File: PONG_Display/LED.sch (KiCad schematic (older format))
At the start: 4 parts, among them J1 LED_Display_Conn, U1 PC817

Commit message: layout v1
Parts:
- C1: footprint Capacitor_SMD:C_1206_3216Metric_Pad1.42x1.75mm_HandSolder -> Capacitor_SMD:C_0603_1608Metric_Pad1.05x0.95mm_HandSolder
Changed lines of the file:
@@
 EESchema Schematic File Version 4
-LIBS:PONG_Display-cache
 EELAYER 30 0
 EELAYER END
@@
 F 0 "C1" H 3515 2996 50  0000 L CNN
 F 1 "100n" H 3515 2905 50  0000 L CNN
-F 2 "Capacitor_SMD:C_1206_3216Metric_Pad1.42x1.75mm_HandSolder" H 3438 2800 50  0001 C CNN
+F 2 "Capacitor_SMD:C_0603_1608Metric_Pad1.05x0.95mm_HandSolder" H 3438 2800 50  0001 C CNN
 F 3 "~" H 3400 2950 50  0001 C CNN
 	1    3400 2950

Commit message: l
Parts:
- R1: footprint Resistor_SMD:R_1206_3216Metric_Pad1.42x1.75mm_HandSolder -> Resistor_SMD:R_0603_1608Metric_Pad1.05x0.95mm_HandSolder
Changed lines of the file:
@@
 F 0 "R1" V 1993 2550 50  0000 C CNN
 F 1 "180R" V 2084 2550 50  0000 C CNN
-F 2 "Resistor_SMD:R_1206_3216Metric_Pad1.42x1.75mm_HandSolder" V 2130 2550 50  0001 C CNN
+F 2 "Resistor_SMD:R_0603_1608Metric_Pad1.05x0.95mm_HandSolder" V 2130 2550 50  0001 C CNN
 F 3 "~" H 2200 2550 50  0001 C CNN
 	1    2200 2550

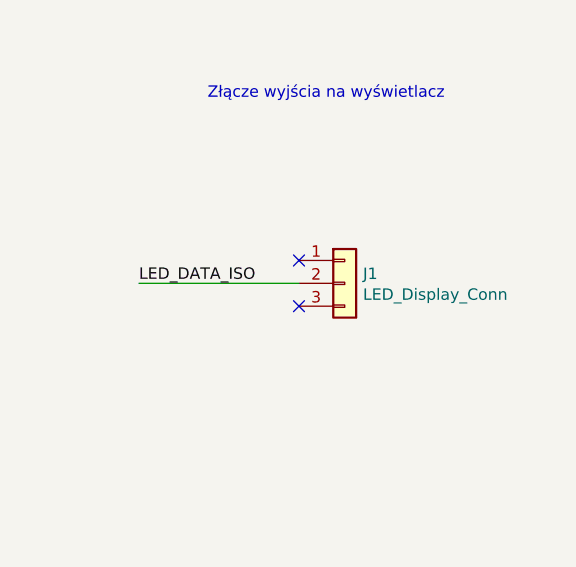
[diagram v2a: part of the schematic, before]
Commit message: layout4
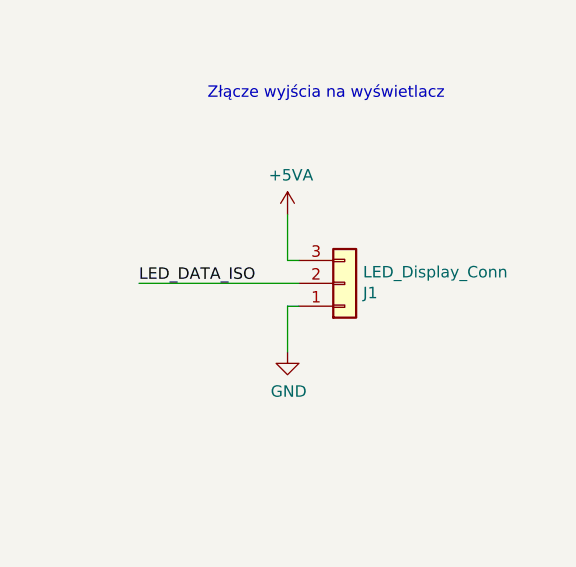
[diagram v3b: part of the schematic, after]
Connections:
- net GND: now also J1.1 (Pin_1)
- net +5VA: now reaches J1.3 (Pin_3)
- no-connect marks 2 -> 0
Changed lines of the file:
@@
 F 3 "~" H 8850 2800 50  0001 C CNN
 	1    8850 2800
-	1    0    0    -1
+	1    0    0    1
 $EndComp
 Text Notes 7750 7500 0    50   ~ 0
@@
 	1    0    0    -1
 $EndComp
-NoConn ~ 8650 2700
-NoConn ~ 8650 2900
+$Comp
+L power:GND #PWR0109
+U 1 1 5EB33F3E
+P 8600 3100
+F 0 "#PWR0109" H 8600 2850 50  0001 C CNN
+F 1 "GND" H 8605 2927 50  0000 C CNN
+F 2 "" H 8600 3100 50  0001 C CNN
+F 3 "" H 8600 3100 50  0001 C CNN
+	1    8600 3100
+	1    0    0    -1
+$EndComp
+Wire Wire Line
+	8600 2500 8600 2700
+Wire Wire Line
+	8600 2700 8650 2700
+Wire Wire Line
+	8600 3100 8600 2900
+Wire Wire Line
+	8600 2900 8650 2900
+$Comp
+L power:+5VA #PWR0110
+U 1 1 5EA4877F
+P 8600 2500
+F 0 "#PWR0110" H 8600 2350 50  0001 C CNN
+F 1 "+5VA" H 8615 2673 50  0000 C CNN
+F 2 "" H 8600 2500 50  0001 C CNN
+F 3 "" H 8600 2500 50  0001 C CNN
+	1    8600 2500
+	1    0    0    -1
+$EndComp
 $EndSCHEMATC

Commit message: laayout6
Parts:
- J1: footprint TerminalBlock:TerminalBlock_bornier-3_P5.08mm -> TerminalBlock_RND:TerminalBlock_RND_205-00002_1x03_P5.00mm_Horizontal
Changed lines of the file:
@@
 F 0 "J1" H 8930 2842 50  0000 L CNN
 F 1 "LED_Display_Conn" H 8930 2751 50  0000 L CNN
-F 2 "TerminalBlock:TerminalBlock_bornier-3_P5.08mm" H 8850 2800 50  0001 C CNN
+F 2 "TerminalBlock_RND:TerminalBlock_RND_205-00002_1x03_P5.00mm_Horizontal" H 8850 2800 50  0001 C CNN
 F 3 "~" H 8850 2800 50  0001 C CNN
 	1    8850 2800
